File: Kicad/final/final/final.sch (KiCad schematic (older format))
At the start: 67 parts, among them J1 54-00164, J2 Backup_If_Motor_driver_dont_w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, J3 AC_IN, J4 AC_OUT, K1 SRD-S-112DM(F-11), Q1 PJE8408_R1_00001, Q2 PJE8408_R1_00001, Q3 PJE8408_R1_00001, SW16 SW, SW17 SW, SW18 SW, SW19 SW, U1 SN74LVC2G06DCKR, U2 L2293QTR, U3 PSK-20D-12, U4 SN74AHCT595N, U5 esp32_dev, U6 EE2-5NU, U7 EE2-5NU

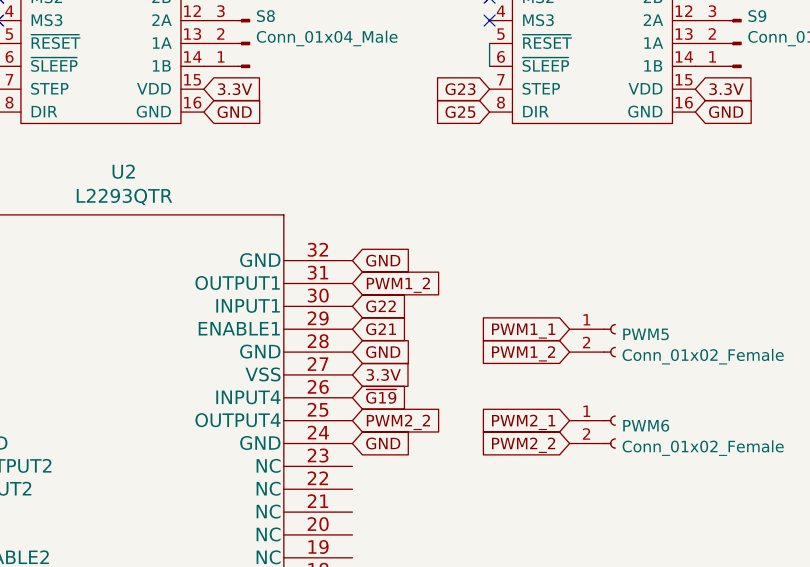
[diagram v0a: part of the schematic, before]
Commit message: Did more
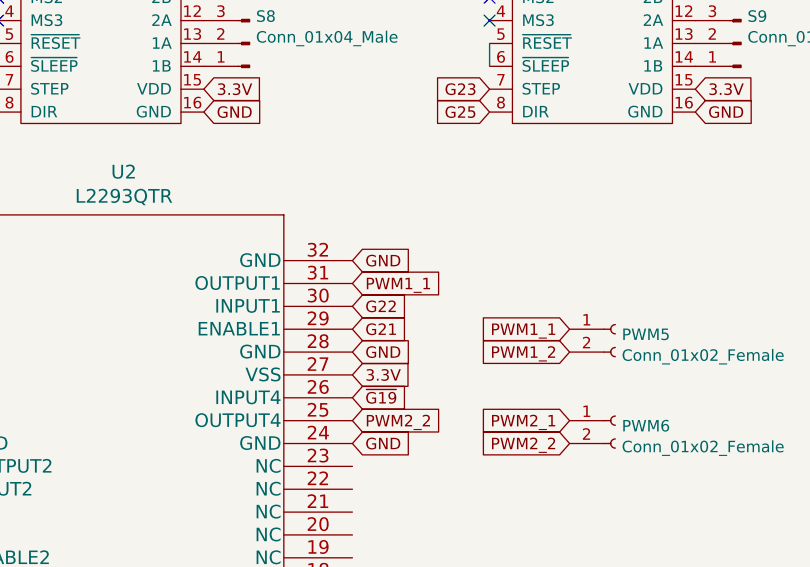
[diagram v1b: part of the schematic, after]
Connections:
- net PWM1_1: now also U2.31 (OUTPUT1)
- net PWM1_2: no longer U2.31 (OUTPUT1)
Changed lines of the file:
@@
 $EndComp
 Text GLabel 5100 5750 2    50   Input ~ 0
-PWM1_2
+PWM1_1
 Text GLabel 3100 6550 0    50   Input ~ 0
 PWM1_2
